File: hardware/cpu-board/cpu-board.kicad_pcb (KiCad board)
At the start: 2 copper layers, 100 x 80 mm, 44 parts, among them CON1 BARREL_JACK, P1 CTRL1, P2 CTRL2, P3 DATA, P4 IO, P5 ADDR1, P6 ADDR2, SW1 RESET, U1 WD65C02, U2 AT28C256, U3 74HC132, U4 CY7C199, U5 MXO45HS, U6 7805, U7 4012, U8 4012, U9 74HC138

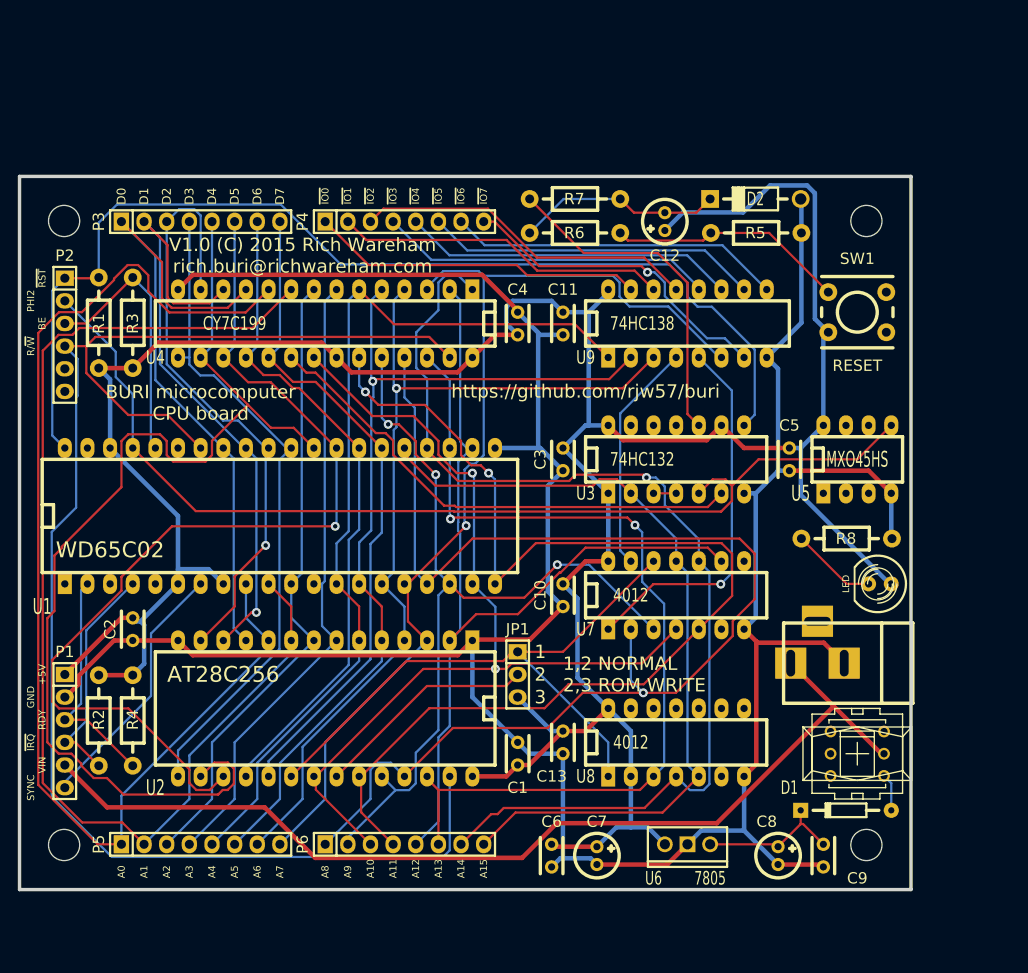
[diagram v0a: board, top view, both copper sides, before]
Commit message: add v3 hardware
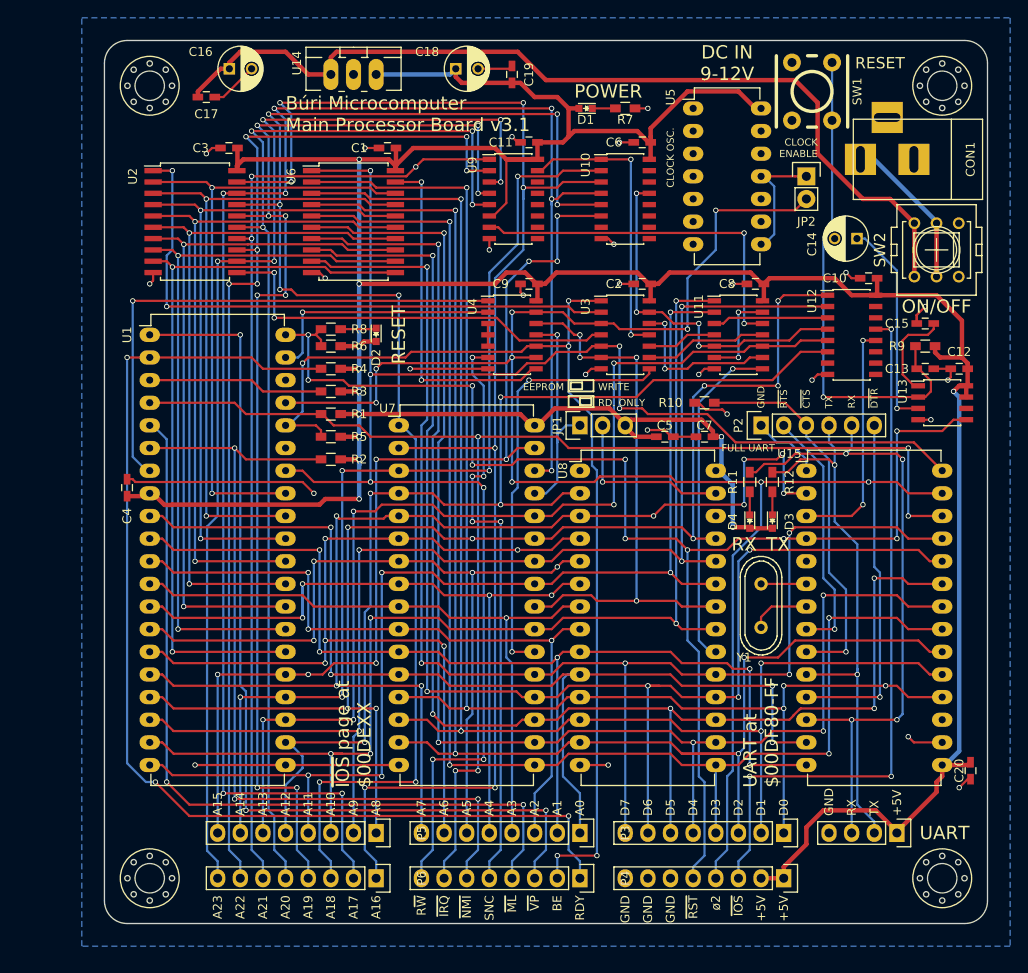
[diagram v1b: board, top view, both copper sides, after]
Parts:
- removed Outl: EuroBoard_halb_Type-I_100mmX80mm_holes, EuroBoard_Outline:EuroBoard_halb_Type-I_100mmX80mm_holes
- removed S1: PWR, switch-misc-PVA2F
- added C14: 1µ, Capacitors_ThroughHole:C_Radial_D5_L6_P2.5, F.Cu at (181.6, 74.3)
- added C15: 100n, Capacitors_SMD:C_0603_HandSoldering, F.Cu at (189.2, 83.8)
- added C16: 1µ, Capacitors_ThroughHole:C_Radial_D5_L6_P2.5, F.Cu at (111.2, 55.2)
- added C17: 100n, Capacitors_SMD:C_0603_HandSoldering, F.Cu at (108.6, 58.4)
- added C18: 1µ, Capacitors_ThroughHole:C_Radial_D5_L6_P2.5, F.Cu at (136.6, 55.2)
- added C19: 100n, Capacitors_SMD:C_0603_HandSoldering, F.Cu at (142.9, 55.9)
- added C20: 100n, Capacitors_SMD:C_0603_HandSoldering, F.Cu at (194.3, 134.0)
- added D4: RX, LEDs:LED_0603, F.Cu at (169.5, 106.0)
- added JP2: Jumper_NC_Small, Pin_Headers:Pin_Header_Straight_1x02, F.Cu at (175.9, 67.3)
- added P7: CTRL2, Pin_Headers:Pin_Header_Straight_1x08, F.Cu at (173.4, 146.1)
- added P8: UARTMINI, Pin_Headers:Pin_Header_Straight_1x04, F.Cu at (186.1, 141.0)
- added R10: 330, Resistors_SMD:R_0603_HandSoldering, F.Cu at (164.5, 92.7)
- added R11: 330, Resistors_SMD:R_0603_HandSoldering, F.Cu at (172.1, 101.6)
- added R12: 330, Resistors_SMD:R_0603_HandSoldering, F.Cu at (169.5, 101.6)
- added R9: 330, Resistors_SMD:R_0603_HandSoldering, F.Cu at (189.2, 86.4)
- added SW2: ON/OFF, buri3:switch-misc-PVA2R, F.Cu at (190.5, 75.6)
- added U10: 74HC138, Housings_SOIC:SOIC-16_3.9x9.9mm_Pitch1.27mm, F.Cu at (155.6, 69.8)
- added U11: 74HC00, Housings_SOIC:SOIC-14_3.9x8.7mm_Pitch1.27mm, F.Cu at (168.3, 85.1)
- added U12: 74HC138, Housings_SOIC:SOIC-16_3.9x9.9mm_Pitch1.27mm, F.Cu at (181.0, 85.1)
- added U13: TL7705A, Housings_SOIC:SOIC-8_3.9x4.9mm_Pitch1.27mm, F.Cu at (191.1, 92.7)
- added U14: 7805, TO_SOT_Packages_THT:TO-220_Neutral123_Vertical_LargePads, F.Cu at (125.1, 55.9)
- added U15: W65C51, Housings_DIP:DIP-28_W15.24mm_LongPads, F.Cu at (175.9, 100.3)
- added W1: MOUNTING, buri3:M3_MOUNT, F.Cu at (102.2, 146.1)
- added W2: MOUNTING, buri3:M3_MOUNT, F.Cu at (191.1, 146.1)
- added W3: MOUNTING, buri3:M3_MOUNT, F.Cu at (191.1, 57.1)
- added W4: MOUNTING, buri3:M3_MOUNT, F.Cu at (102.2, 57.1)
- added Y1: 1.8432M, Crystals:Crystal_HC49-U_Vertical, F.Cu at (170.8, 115.5)
- C1, C10, C11, C13, C2, C3, C4, C5, C9: value 10nF -> 100n; footprint Capacitors_ThroughHole:Capacitor4x3RM2.5 -> Capacitors_SMD:C_0603_HandSoldering
- C12, C8: value 4.7uF -> 100n; footprint Capacitors_Elko_ThroughHole:Elko_vert_DM5_RM2 -> Capacitors_SMD:C_0603_HandSoldering
- C6: value 4.7uF -> 100n; footprint Capacitors_ThroughHole:Capacitor4x3RM2.5 -> Capacitors_SMD:C_0603_HandSoldering
- C7: value 10nF -> 100n; footprint Capacitors_Elko_ThroughHole:Elko_vert_DM5_RM2 -> Capacitors_SMD:C_0603_HandSoldering
- CON1: value BARREL_JACK -> POWER_IN
- D1: value 1N4001 -> PWR; footprint Diodes_ThroughHole:Diode_DO-35_SOD27_Horizontal_RM10 -> LEDs:LED_0603
- D2: value 1N4148 -> RST; footprint Diodes_ThroughHole:Diode_DO-41_SOD81_Horizontal_RM10 -> LEDs:LED_0603
- D3: value LED -> TX; footprint LEDs:LED-5MM -> LEDs:LED_0603
- JP1: value ROM PROGRAMMABLE -> ROMWRITE
- P1: value CTRL1 -> D0..D7; footprint Socket_Strips:Socket_Strip_Straight_1x06 -> Pin_Headers:Pin_Header_Straight_1x08
- P2: value CTRL2 -> UART; footprint Socket_Strips:Socket_Strip_Straight_1x06 -> Pin_Headers:Pin_Header_Straight_1x06
- P3: value DATA -> A0..A7; footprint Socket_Strips:Socket_Strip_Straight_1x08 -> Pin_Headers:Pin_Header_Straight_1x08
- P4: value IO -> CTRL1; footprint Socket_Strips:Socket_Strip_Straight_1x08 -> Pin_Headers:Pin_Header_Straight_1x08
- P5: value ADDR1 -> A8..A15; footprint Socket_Strips:Socket_Strip_Straight_1x08 -> Pin_Headers:Pin_Header_Straight_1x08
- P6: value ADDR2 -> A16..A23; footprint Socket_Strips:Socket_Strip_Straight_1x08 -> Pin_Headers:Pin_Header_Straight_1x08
- R1, R2, R3, R4, R6, R7: value 10K -> 330; footprint Resistors_ThroughHole:Resistor_Horizontal_RM10mm -> Resistors_SMD:R_0603_HandSoldering
- R5: value 47K -> 330; footprint Resistors_ThroughHole:Resistor_Horizontal_RM10mm -> Resistors_SMD:R_0603_HandSoldering
- R8: footprint Resistors_ThroughHole:Resistor_Horizontal_RM10mm -> Resistors_SMD:R_0603_HandSoldering
- SW1: footprint IHeartKiCad:SW_M6_PTH -> buri3:SW_M6_PTH
- U1: value WD65C02 -> W65C816; footprint Sockets_DIP:DIP-40__600_ELL -> Housings_DIP:DIP-40_W15.24mm_LongPads
- U2: value AT28C256 -> 74HC573; footprint Sockets_DIP:DIP-28__600_ELL -> Housings_SOIC:SOIC-20_7.5x12.8mm_Pitch1.27mm
- U3: value 74HC132 -> 74HC04; footprint Sockets_DIP:DIP-14__300_ELL -> Housings_SOIC:SOIC-14_3.9x8.7mm_Pitch1.27mm
- U4: value CY7C199 -> 74HC00; footprint Sockets_DIP:DIP-28__300_ELL -> Housings_SOIC:SOIC-14_3.9x8.7mm_Pitch1.27mm
- U5: value MXO45HS -> CLOCK; footprint Sockets_DIP:DIP-8__300_ELL -> Housings_DIP:DIP-14_W7.62mm_LongPads
- U6: value 7805 -> 74HC245; footprint Discret:LM78XXV -> Housings_SOIC:SOIC-20_7.5x12.8mm_Pitch1.27mm
- U7: value 4012 -> AS6C4008; footprint Sockets_DIP:DIP-14__300_ELL -> Housings_DIP:DIP-32_W15.24mm_LongPads
- U8: value 4012 -> AT28C64B; footprint Sockets_DIP:DIP-14__300_ELL -> Housings_DIP:DIP-28_W15.24mm_LongPads
- U9: footprint Sockets_DIP:DIP-16__300_ELL -> Housings_SOIC:SOIC-16_3.9x9.9mm_Pitch1.27mm
- moved D1 84.0 mm to (151.1, 59.7)
- moved P1 81.5 mm to (173.4, 141.0)
- moved P3 80.7 mm to (150.5, 141.0), turned to 270 degrees
- moved C6 79.4 mm to (157.5, 63.5), turned to 180 degrees
- moved U6 79.3 mm to (125.1, 72.4), turned to 0 degrees
- moved P2 78.8 mm to (170.8, 95.2), turned to 90 degrees
- moved P4 76.2 mm to (150.5, 146.1), turned to 270 degrees
- moved C9 71.0 mm to (144.8, 79.4), turned to 180 degrees
- moved C1 70.7 mm to (128.9, 64.1), turned to 180 degrees
- moved C2 68.3 mm to (157.5, 79.4), turned to 180 degrees
- moved C8 64.2 mm to (170.2, 79.4), turned to 180 degrees
- moved R8 62.4 mm to (122.6, 84.5), turned to 180 degrees
- moved C13 57.5 mm to (189.2, 88.9), turned to 0 degrees
- moved CON1 57.1 mm to (188.2, 65.4)
- moved U2 56.5 mm to (107.3, 72.4), turned to 0 degrees
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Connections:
- C12 pad 2: Net-(C12-Pad2) -> GND
- C13 pad 1: +5V -> Net-(C13-Pad1)
- C8 pad 1: Net-(C8-Pad1) -> +5V
- C9 pad 1: Net-(C8-Pad1) -> +5V
- CON1 pad 1: VIN -> Net-(CON1-Pad1)
- CON1 pad 3: (no net) -> Net-(CON1-Pad3)
- D1 pad 2: Net-(C8-Pad1) -> +5V
- D2 pad 1: GND -> Net-(D2-Pad1)
- D2 pad 2: Net-(C12-Pad2) -> +5V
- D3 pad 1: +5V -> Net-(D3-Pad1)
- D3 pad 2: Net-(D3-Pad2) -> +5V
- JP1 pad 1: /Address Decode/~ROMSEL -> /~MEMWE
- JP1 pad 2: /~ROMOE -> /~ROMWE
- P1 pad 1: +5V -> /ACIA/D0
- P1 pad 2: GND -> /ACIA/D1
- P1 pad 3: RDY -> /ACIA/D2
- P1 pad 4: ~IRQ -> /ACIA/D3
- P1 pad 5: VIN -> /ACIA/D4
- P1 pad 6: SYNC -> /ACIA/D5
- P2 pad 1: ~RST -> GND
- P2 pad 2: PHI2 -> /ACIA/~RTS
- P2 pad 3: BE -> /ACIA/~CTS
- P2 pad 4: R/~W -> /ACIA/TX
- P2 pad 5: (no net) -> /ACIA/RX
- P2 pad 6: (no net) -> /ACIA/~DTR
- P3 pad 1: D0 -> /ACIA/RS0
- P3 pad 2: D1 -> /ACIA/RS1
- P3 pad 3: D2 -> /A2
- P3 pad 4: D3 -> /A3
- P3 pad 5: D4 -> /A4
- P3 pad 6: D5 -> /A5
- P3 pad 7: D6 -> /A6
- P3 pad 8: D7 -> /ACIA/CS0
- P4 pad 1: ~IO0 -> /RDY
- P4 pad 2: ~IO1 -> /BE
- P4 pad 3: ~IO2 -> /~VP
- P4 pad 4: ~IO3 -> /~ML
- P4 pad 5: ~IO4 -> /SYNC
- P4 pad 6: ~IO5 -> /~NMI
- P4 pad 7: ~IO6 -> /ACIA/~IRQ
- P4 pad 8: ~IO7 -> /ACIA/R/~W
- P5 pad 1: A0 -> /Address decode/A8
- P5 pad 2: A1 -> /Address decode/A9
- P5 pad 3: A2 -> /Address decode/A10
- P5 pad 4: A3 -> /Address decode/A11
- P5 pad 5: A4 -> /Address decode/A12
- P5 pad 6: A5 -> /Address decode/A13
- P5 pad 7: A6 -> /Address decode/A14
- P5 pad 8: A7 -> /Address decode/A15
- P6 pad 1: A8 -> /Address decode/A16
- P6 pad 2: A9 -> /Address decode/A17
- P6 pad 3: A10 -> /Address decode/A18
- P6 pad 4: A11 -> /Address decode/A19
- P6 pad 5: A12 -> /Address decode/A20
- P6 pad 6: A13 -> /Address decode/A21
- P6 pad 7: A14 -> /Address decode/A22
- P6 pad 8: A15 -> /Address decode/A23
- R1 pad 2: ~RST -> /ACIA/~IRQ
- R2 pad 2: ~IRQ -> /~NMI
- R3 pad 2: BE -> /~ABORT
- R4 pad 2: RDY -> /RDY
- R5 pad 1: Net-(R5-Pad1) -> +5V
- R5 pad 2: GND -> /BE
- R6 pad 1: Net-(C12-Pad2) -> +5V
- R6 pad 2: Net-(R5-Pad1) -> /Reset & power/~RESET
- R7 pad 1: Net-(R7-Pad1) -> GND
- R7 pad 2: Net-(C12-Pad2) -> Net-(D1-Pad1)
- R8 pad 1: Net-(D3-Pad2) -> Net-(D2-Pad1)
- R8 pad 2: GND -> /Reset & power/~RESET
- SW1 pad 1: Net-(R5-Pad1) -> GND
- SW1 pad 2: +5V -> Net-(C13-Pad1)
- U1 pad 1: (no net) -> /~VP
- U1 pad 10: A1 -> /ACIA/RS1
- U1 pad 11: A2 -> /A2
- U1 pad 12: A3 -> /A3
- U1 pad 13: A4 -> /A4
- U1 pad 14: A5 -> /A5
- U1 pad 15: A6 -> /A6
- U1 pad 16: A7 -> /ACIA/CS0
- U1 pad 17: A8 -> /Address decode/A8
- U1 pad 18: A9 -> /Address decode/A9
- U1 pad 19: A10 -> /Address decode/A10
- U1 pad 2: RDY -> /RDY
- U1 pad 20: A11 -> /Address decode/A11
- U1 pad 22: A12 -> /Address decode/A12
- U1 pad 23: A13 -> /Address decode/A13
- U1 pad 24: A14 -> /Address decode/A14
- U1 pad 25: A15 -> /Address decode/A15
- U1 pad 26: D7 -> /BA7
- U1 pad 27: D6 -> /BA6
- U1 pad 28: D5 -> /BA5
- U1 pad 29: D4 -> /BA4
- U1 pad 3: (no net) -> /~ABORT
- U1 pad 30: D3 -> /BA3
- U1 pad 31: D2 -> /BA2
- U1 pad 32: D1 -> /BA1
- U1 pad 33: D0 -> /BA0
- U1 pad 34: R/~W -> /ACIA/R/~W
- U1 pad 35: (no net) -> Net-(U1-Pad35)
- U1 pad 36: BE -> /BE
- U1 pad 37: PHI2 -> /ACIA/PHI2
- U1 pad 38: +5V -> Net-(U1-Pad38)
- U1 pad 39: (no net) -> /VDA
- U1 pad 4: ~IRQ -> /ACIA/~IRQ
- U1 pad 40: ~RST -> /Reset & power/~RESET
- U1 pad 5: (no net) -> /~ML
- U1 pad 6: +5V -> /~NMI
- U1 pad 7: SYNC -> /VPA
- U1 pad 9: A0 -> /ACIA/RS0
- U2 pad 1: GND -> Net-(U2-Pad1)
- U2 pad 10: A0 -> GND
- U2 pad 11: D0 -> Net-(U2-Pad11)
- U2 pad 12: D1 -> /Address decode/A23
- U2 pad 13: D2 -> /Address decode/A22
- U2 pad 14: GND -> /Address decode/A21
- U2 pad 15: D3 -> /Address decode/A20
- U2 pad 16: D4 -> /Address decode/A19
- U2 pad 17: D5 -> /Address decode/A18
- U2 pad 18: D6 -> /Address decode/A17
- U2 pad 19: D7 -> /Address decode/A16
- U2 pad 2: A12 -> /BA0
- U2 pad 20: /Address Decode/~ROMSEL -> +5V
- U2 pad 3: A7 -> /BA1
- U2 pad 4: A6 -> /BA2
- U2 pad 5: A5 -> /BA3
- U2 pad 6: A4 -> /BA4
- U2 pad 7: A3 -> /BA5
- U2 pad 8: A2 -> /BA6
- U2 pad 9: A1 -> /BA7
- U3 pad 1: +5V -> /BE
- U3 pad 10: Net-(R7-Pad1) -> /Address decode/LOADDR
- U3 pad 11: (no net) -> /Address decode/~LOADDR
- U3 pad 12: (no net) -> /Address decode/RAMHOLE
- U3 pad 13: (no net) -> /Address decode/~RAMHOLE
- U3 pad 2: A15 -> Net-(U2-Pad1)
- U3 pad 3: Net-(U3-Pad3) -> /ACIA/PHI2
- U3 pad 4: Net-(U3-Pad3) -> Net-(U2-Pad11)
- U3 pad 5: PHI2 -> /ACIA/R/~W
- U3 pad 6: /~RAMCE -> /~R~/W
- U3 pad 8: ~RST -> /~RAMSEL
- U3 pad 9: +5V -> /Address decode/RAMSEL
- U4 pad 1: A14 -> /VPA
- U4 pad 10: A0 -> /BE
- U4 pad 11: D0 -> /~MEMWE
- U4 pad 12: D1 -> /~R~/W
- U4 pad 13: D2 -> /ACIA/PHI2
- U4 pad 14: GND -> +5V
- U4 pad 2: A12 -> /VDA
- U4 pad 3: A7 -> Net-(U4-Pad3)
- U4 pad 4: A6 -> Net-(U4-Pad3)
- U4 pad 5: A5 -> Net-(U4-Pad3)
- U4 pad 6: A4 -> /SYNC
- U4 pad 7: A3 -> GND
- U4 pad 8: A2 -> Net-(U4-Pad8)
- U4 pad 9: A1 -> /ACIA/PHI2
- U5 pad 5: PHI2 -> (no net)
- U5 pad 7: (no net) -> GND
- U5 pad 8: +5V -> Net-(JP2-Pad1)
- U7 pad 1: Net-(U7-Pad1) -> /Address decode/A18
- U7 pad 10: A14 -> /A2
- U7 pad 11: A15 -> /ACIA/RS1
- U7 pad 12: /Address Decode/~ROMSEL -> /ACIA/RS0
- U7 pad 13: Net-(U7-Pad13) -> /ACIA/D0
- U7 pad 14: +5V -> /ACIA/D1
- U7 pad 2: A8 -> /Address decode/A16
- U7 pad 3: A9 -> /Address decode/A14
- U7 pad 4: A10 -> /Address decode/A12
- U7 pad 5: A11 -> /ACIA/CS0
- U7 pad 6: (no net) -> /A6
- U7 pad 7: GND -> /A5
- U7 pad 8: (no net) -> /A4
- U7 pad 9: A12 -> /A3
- U8 pad 1: /Address Decode/~ROMSEL -> Net-(U8-Pad1)
- U8 pad 10: (no net) -> /ACIA/RS0
- U8 pad 11: (no net) -> /ACIA/D0
- U8 pad 12: (no net) -> /ACIA/D1
- U8 pad 13: (no net) -> /ACIA/D2
- U8 pad 14: +5V -> GND
- U8 pad 2: +5V -> /Address decode/A12
- U8 pad 3: A13 -> /ACIA/CS0
- U8 pad 4: A14 -> /A6
- U8 pad 5: A15 -> /A5
- U8 pad 6: (no net) -> /A4
- U8 pad 7: GND -> /A3
- U8 pad 8: (no net) -> /A2
- U8 pad 9: (no net) -> /ACIA/RS1
- U9 pad 1: A4 -> /Address decode/A21
- U9 pad 10: ~IO5 -> Net-(U9-Pad10)
- U9 pad 11: ~IO4 -> Net-(U9-Pad11)
- U9 pad 12: ~IO3 -> Net-(U9-Pad12)
- U9 pad 13: ~IO2 -> Net-(U9-Pad13)
- U9 pad 14: ~IO1 -> Net-(U9-Pad14)
- U9 pad 15: ~IO0 -> /Address decode/~LOADDR
- U9 pad 2: A5 -> /Address decode/A22
- U9 pad 3: A6 -> /Address decode/A23
- U9 pad 4: Net-(U7-Pad13) -> /Address decode/A19
- U9 pad 5: Net-(U7-Pad1) -> /Address decode/A20
- U9 pad 6: A7 -> +5V
- U9 pad 7: ~IO7 -> /Address decode/~HIADDR
- U9 pad 9: ~IO6 -> Net-(U9-Pad9)
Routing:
- net /ACIA/PHI2: track 0.00 -> 193.2 mm, vias 0 -> 9
- net GND: track 318.9 -> 125.9 mm, vias 0 -> 27
- net /ACIA/R/~W: track 0.00 -> 189.9 mm, vias 0 -> 8
- net /Address decode/A17: track 0.00 -> 187.8 mm, vias 0 -> 8
- net R/~W: track 172.3 -> 0.00 mm
- net /Address decode/A16: track 0.00 -> 167.7 mm, vias 0 -> 7
- net /ACIA/D2: track 0.00 -> 166.9 mm, vias 0 -> 4
- net /Address decode/A18: track 0.00 -> 163.8 mm, vias 0 -> 8
- net /ACIA/D1: track 0.00 -> 158.8 mm, vias 0 -> 4
- net /ACIA/D3: track 0.00 -> 156.9 mm, vias 0 -> 4
- net /ACIA/D4: track 0.00 -> 156.6 mm, vias 0 -> 5
- net /ACIA/D6: track 0.00 -> 156.2 mm, vias 0 -> 5
- net /ACIA/D5: track 0.00 -> 155.8 mm, vias 0 -> 5
- net /ACIA/D0: track 0.00 -> 155.7 mm, vias 0 -> 5
- net /Reset & power/~RESET: track 0.00 -> 155.0 mm, vias 0 -> 10
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- removed copper zone on F.Cu, net GND
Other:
- board size 100 x 80 mm -> 99.1 x 99.1 mm
- net class Default: clearance 0.254 -> 0.2; trace_width 0.254 -> 0.25; via_dia 1 -> 0.6; via_drill 0.8 -> 0.4
- net class Power removed
- rule trace_clearance: 0.254 -> 0.2
- rule trace_min: 0.254 -> 0.2
- rule via_min_drill: 0.5 -> 0.3
- rule via_min_size: 0.8 -> 0.4
- board text added: "A16"
- board text added: "A17"
- board text added: "A18"
- board text added: "A19"
- board text added: "A20"
- board text added: "A21"
- board text added: "A22"
- board text added: "A23"
- board text added: "Búri Microcomputer Main Processor Board v3.1"
- board text added: "Búri Microcomputer Main Processor Board v3.1 ©2016 Rich Wareham rich.buri@richwareham.com CC BY-NC-SA 4.0"
- board text added: "CLOCK ENABLE"
- board text added: "CLOCK OSC."
- board text added: "DC IN 9-12V"
- board text added: "EEPROM"
- board text added: "FULL UART"
- board text added: "POWER"
- board text added: "RD. ONLY"
- board text added: "RESET"
- board text added: "RX"
- board text added: "R~W"
- board text added: "SNC"
- board text added: "TX"
- board text added: "UART"
- board text added: "UART at $00DF80-FF"
- board text added: "WRITE"
- board text added: "~CTS"
- board text added: "~DTR"
- board text added: "~IOS"
- board text added: "~IOS~ page at $00DEXX"
- board text added: "~ML"
- board text added: "~NMI"
- board text added: "~RTS"
- board text added: "~VP"
- board text added: "ø2"
- board text removed: "1"
- board text removed: "1,2 NORMAL 2,3 ROM WRITE"
- board text removed: "2"
- board text removed: "3"
- board text removed: "BURI microcomputer CPU board"
- board text removed: "PHI2"
- board text removed: "R/~W"
- board text removed: "SYNC"
- board text removed: "V1.0 (C) 2015 Rich Wareham rich.buri@richwareham.com"
- board text removed: "VIN"
- board text removed: "https://github.com/rjw57/buri"
- board text removed: "~IO0"
- board text removed: "~IO1"
- board text removed: "~IO2"
- board text removed: "~IO3"
- board text removed: "~IO4"
- board text removed: "~IO5"
- board text removed: "~IO6"
- board text removed: "~IO7"
